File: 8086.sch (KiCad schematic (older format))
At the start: 11 parts, among them SW1 SW_Push, U1 8086_Min_Mode, U2 74LS373, U3 74LS373, U4 74LS373, U5 74LS244, U6 74LS245, U7 74LS245

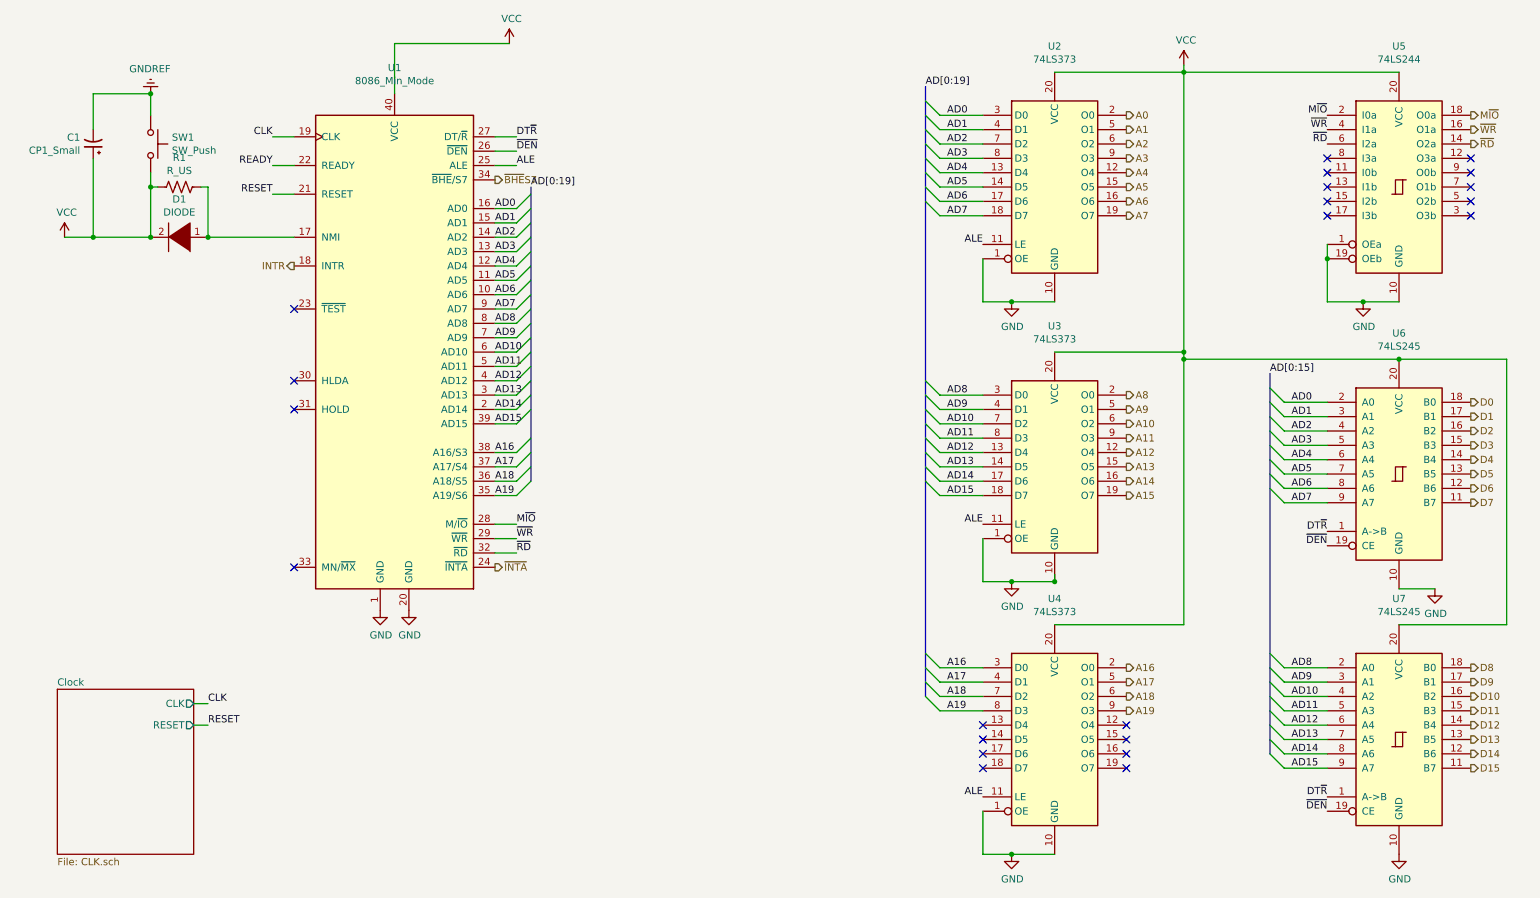
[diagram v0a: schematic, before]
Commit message: Some minor changes
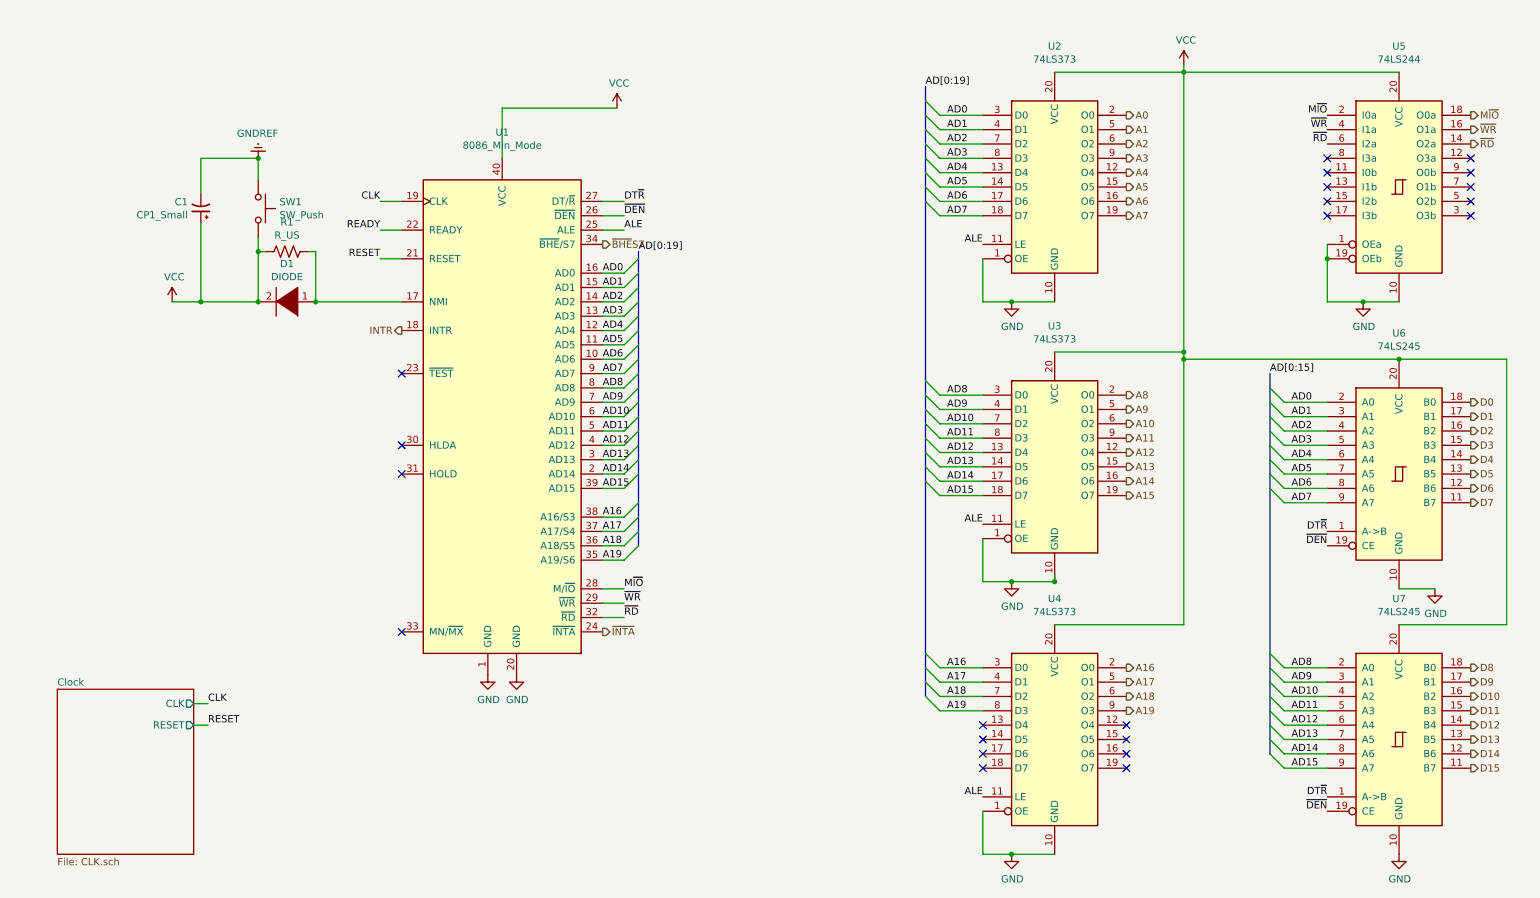
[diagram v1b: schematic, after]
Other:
- moved on the sheet: C1, D1, R1, SW1, U1
